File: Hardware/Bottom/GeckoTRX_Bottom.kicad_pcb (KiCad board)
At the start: 2 copper layers, 120 x 80 mm, 182 parts, among them J1 Jack-DC, J10 Conn_01x04_Female, J11 Conn_01x04_Female, J12 Conn_01x03_Female, J13 Conn_01x03_Female, J14 Conn_01x03_Female, J15 Conn_01x03_Female, J16 Conn_01x03_Female, J17 Conn_01x03_Female, J18 Conn_01x03_Female, J19 Conn_01x03_Female, J2 Conn_Coaxial, J20 Conn_01x03_Female, J21 Conn_01x03_Female, J22 Conn_01x03_Female, J23 Conn_01x03_Female, J24 Conn_01x03_Female, J25 Conn_01x03_Female, J26 Conn_01x03_Female, J27 Conn_01x03_Female, J28 Conn_01x03_Female, J29 Conn_01x03_Female, J3 Conn_02x05_Odd_Even, J30 Conn_01x03_Female, J31 Conn_01x03_Female, J32 Conn_01x03_Female, J4 Conn_02x05_Odd_Even, J5 Conn_01x04_Female, J6 Conn_01x04_Female, J7 Conn_01x04_Female, J8 Conn_01x04_Female, J9 Conn_01x04_Female, K4 G6K-2, T1 MABA-007237-ETC410, U1 TPS562200, U10 74LVC1G17, U11 74HC74D, U2 SN74CBTLV3253, U3 LT6231, U4 OP491-4, U5 MCP23017_ML, U6 Si5351A-B-GM, U7 MCP23017_ML, Y1 25MHz

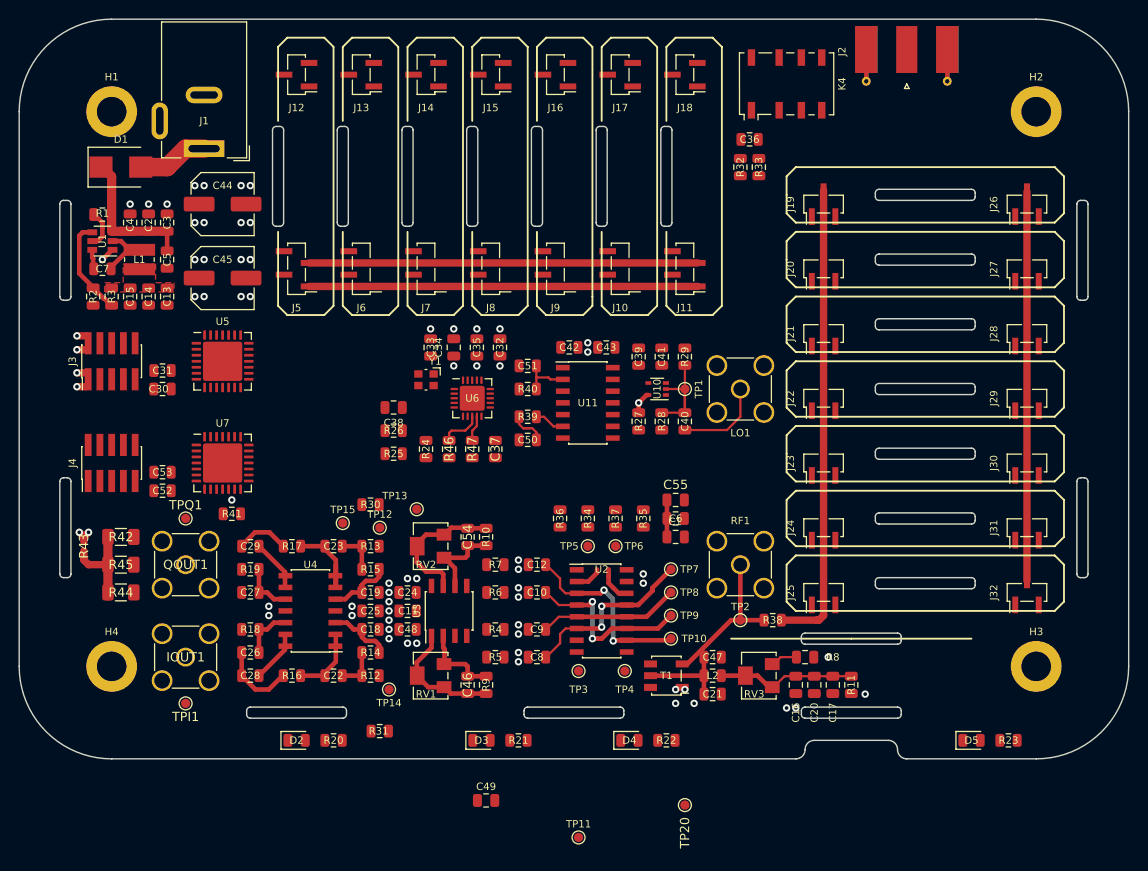
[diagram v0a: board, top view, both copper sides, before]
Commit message: Update
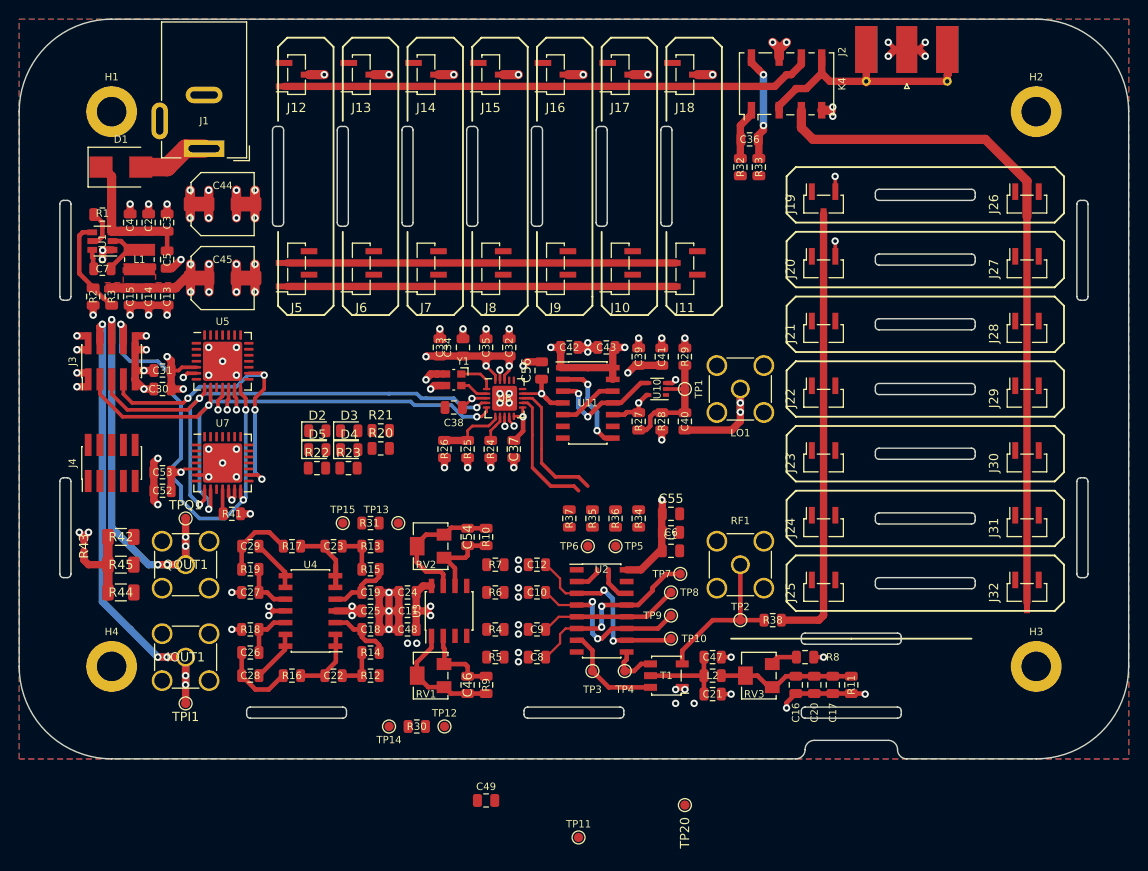
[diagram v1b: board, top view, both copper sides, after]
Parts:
- removed C50, C51: 10p, Capacitor_SMD:C_0805_2012Metric
- removed R39, R40: 1k, Resistor_SMD:R_0805_2012Metric
- removed R46, R47: 10, Resistor_SMD:R_0805_2012Metric
- added C56: 100n, Capacitor_SMD:C_0805_2012Metric, F.Cu at (-3.50, -2.00)
- J10, J11, J5, J6, J7, J8, J9: footprint Connector_PinSocket_1.27mm:PinSocket_1x04_P1.27mm_Vertical_SMD_Pin1Left -> Connector_PinSocket_1.27mm:PinSocket_1x04_P1.27mm_Vertical_SMD_Pin1Right
- J12, J13, J14, J15, J16, J17, J18, J19, J20, J21, J22, J23, J24, J25, J26, J27, J28, J29, J30, J31, J32: footprint Connector_PinSocket_1.27mm:PinSocket_1x03_P1.27mm_Vertical_SMD_Pin1Left -> Connector_PinSocket_1.27mm:PinSocket_1x03_P1.27mm_Vertical_SMD_Pin1Right
- moved D5 77.4 mm to (-27.8, 6.56)
- moved R23 77.2 mm to (-24.4, 8.56)
- moved R22 47.9 mm to (-27.8, 8.56)
- moved D4 43.7 mm to (-24.3, 6.56)
- moved R21 36.7 mm to (-20.9, 4.48)
- moved D3 36.4 mm to (-24.3, 4.52)
- moved D2 33.6 mm to (-27.8, 4.52)
- moved R20 32.0 mm to (-20.9, 6.43)
- moved R30 24.5 mm to (-17.0, 36.5)
- moved TP12 22.6 mm to (-14.0, 36.5)
- moved R31 22.5 mm to (-22.0, 14.5)
- moved R25 8.02 mm to (-11.5, 6.50), turned to 270 degrees
- moved R24 7.00 mm to (-9.00, 6.50)
- moved C38 6.50 mm to (-13.0, 2.00)
- moved R36 6.00 mm to (4.50, 14.0)
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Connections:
- J3 pad 3: /IOC_I2C_SCL -> /IOC_I2C_SDA
- J3 pad 7: /IOC_I2C_SCL -> /IOC_INT_INTA
- J3 pad 8: /IOC_I2C_SCL -> /IOC_~RESET
- R30 pad 2: Net-(R13-Pad2) -> Net-(R12-Pad1)
- R31 pad 2: Net-(R12-Pad1) -> Net-(R13-Pad2)
- U11 pad 12: Net-(C50-Pad2) -> Net-(U11-Pad12)
- U11 pad 2: Net-(C51-Pad2) -> Net-(U11-Pad2)
- U11 pad 5: /Local oscillator/ALTLO_RX_CLKI -> Net-(U11-Pad12)
- U11 pad 6: Net-(R39-Pad1) -> /Local oscillator/ALTLO_RX_CLKQ
- U11 pad 8: /Local oscillator/ALTLO_RX_CLKQ -> Net-(U11-Pad2)
- U11 pad 9: Net-(R40-Pad2) -> /Local oscillator/ALTLO_RX_CLKI
- U5 pad 14: /IOC_I2C_SCL -> /IOC_~RESET
- U5 pad 16: /IOC_I2C_SCL -> /IOC_INT_INTA
- U5 pad 9: /IOC_I2C_SCL -> /IOC_I2C_SDA
- U6 pad 5: /IOC_I2C_SCL -> /IOC_I2C_SDA
- U7 pad 14: /IOC_I2C_SCL -> /IOC_~RESET
- U7 pad 16: /IOC_I2C_SCL -> /IOC_INT_INTA
- U7 pad 9: /IOC_I2C_SCL -> /IOC_I2C_SDA
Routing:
- net GND: track 1.53 -> 151.0 mm, vias 3 -> 90
- net +3V3: track 12.4 -> 129.6 mm, vias 7 -> 35
- net /IOC_I2C_SDA: track 0.00 -> 62.8 mm, vias 0 -> 3
- net /IOC_I2C_SCL: track 0.00 -> 60.0 mm, vias 0 -> 3
- net /Filter/SIG_LP_OUT: track 0.00 -> 57.7 mm
- net Net-(C28-Pad1): track 5.66 -> 60.3 mm, vias 0 -> 5
- net /IOC_~RESET: track 0.00 -> 48.6 mm, vias 0 -> 3
- net Net-(C29-Pad2): track 5.66 -> 51.4 mm, vias 0 -> 5
- net Net-(J2-Pad2): track 0.00 -> 38.2 mm
- net /IOC_INT_INTA: track 0.00 -> 33.8 mm, vias 0 -> 4
- net /Filter/SIG_PRE_IN: track 42.1 -> 74.6 mm
- net /Local oscillator/LO_RX_CLKI: track 0.00 -> 14.5 mm
- net /Local oscillator/LO_RX_CLKQ: track 0.00 -> 13.8 mm
- net Net-(U10-Pad4): track 0.00 -> 12.5 mm, vias 0 -> 2
- net Net-(C36-Pad2): track 0.00 -> 11.7 mm, vias 0 -> 2
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- added copper zone on In2.Cu, net +3V3
- added copper zone on B.Cu, net GND
- added copper zone on F.Cu, net GND
- added copper zone on In1.Cu, net GND
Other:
- copper layers 2 -> 4
